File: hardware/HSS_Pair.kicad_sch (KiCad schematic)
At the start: 20 parts, among them IC3 TPS2HCS08AQPWPRQ1

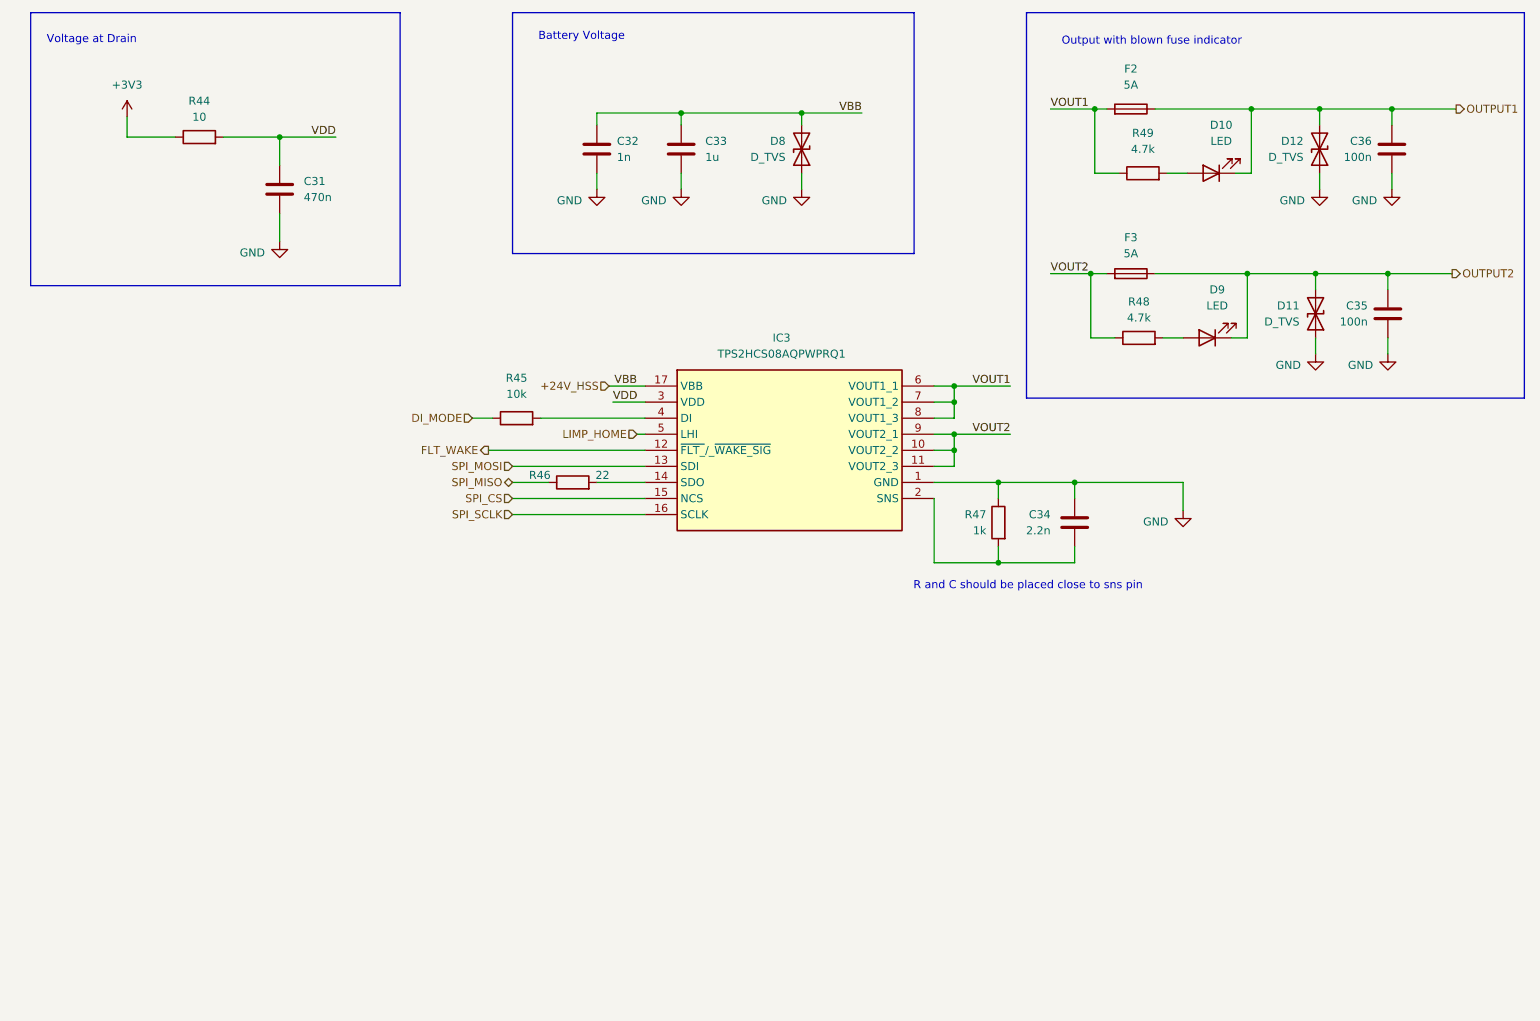
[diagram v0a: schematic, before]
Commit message: what i did during matrices made it pretty
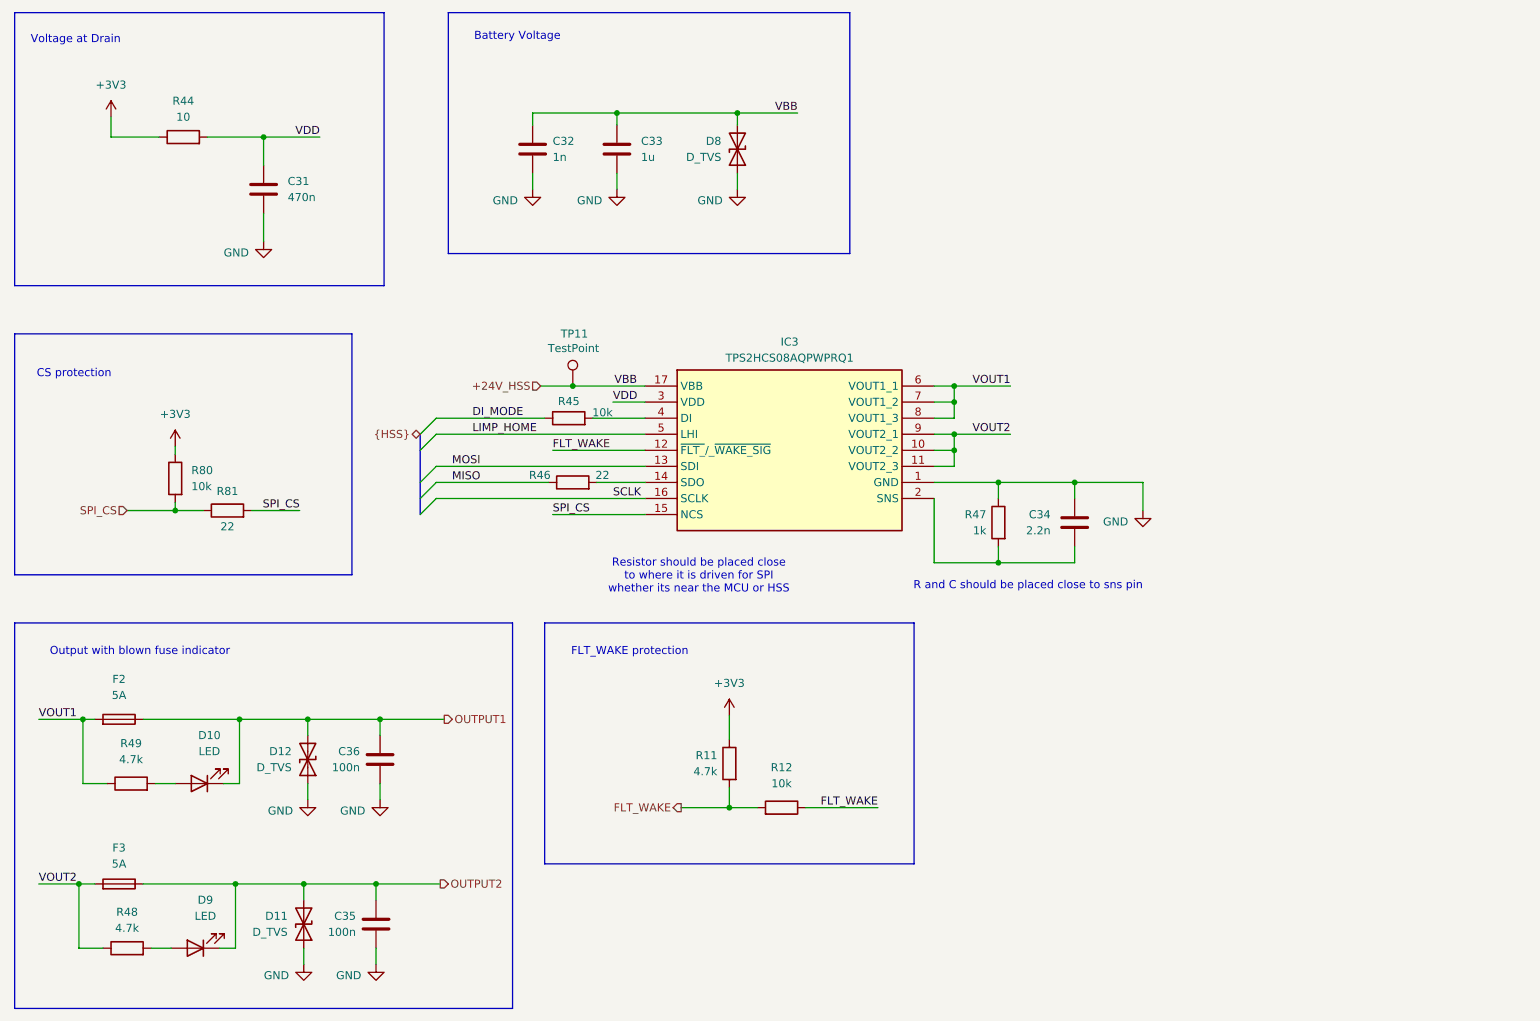
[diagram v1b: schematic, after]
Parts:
- added R11: 4.7k, symbol Device:R
- added R12, R80: 10k, symbol Device:R
- added R81: 22, symbol Device:R
- added TP11: TestPoint, symbol Connector:TestPoint
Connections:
- net +24V_HSS: now also TP11.1
- net +3V3: now also R11.1, R80.1
- net FLT_WAKE: now also R11.2, R12.1, R12.2
- net SPI_CS: now also R80.2, R81.1, R81.2
- net SPI_MISO renamed MISO
- net SPI_MOSI renamed MOSI
- net SPI_SCLK renamed SCLK
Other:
- note added: "CS protection"
- note added: "FLT_WAKE protection"
- note added: "Resistor should be placed close to where it is driven for SPI whether its near the MCU or HSS"
- moved on the sheet: C31, C32, C33, C35, C36, D10, D11, D12, D8, D9, F2, F3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
